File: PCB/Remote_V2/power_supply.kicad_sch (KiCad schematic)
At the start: 69 parts, among them J1 USB_C_Receptacle_USB2.0_16P, J5 USB_C_Receptacle_USB2.0_16P, J6 USB_C_Receptacle_USB2.0_16P, Q1 AO3401A, Q2 AO3401A, Q3 AO3401A, U1 AMS1117-3.3, U3 AMS1117-3.3, U4 AMS1117-3.3, U5 AMS1117-3.3, U7 AMS1117-3.3, U9 AMS1117-3.3

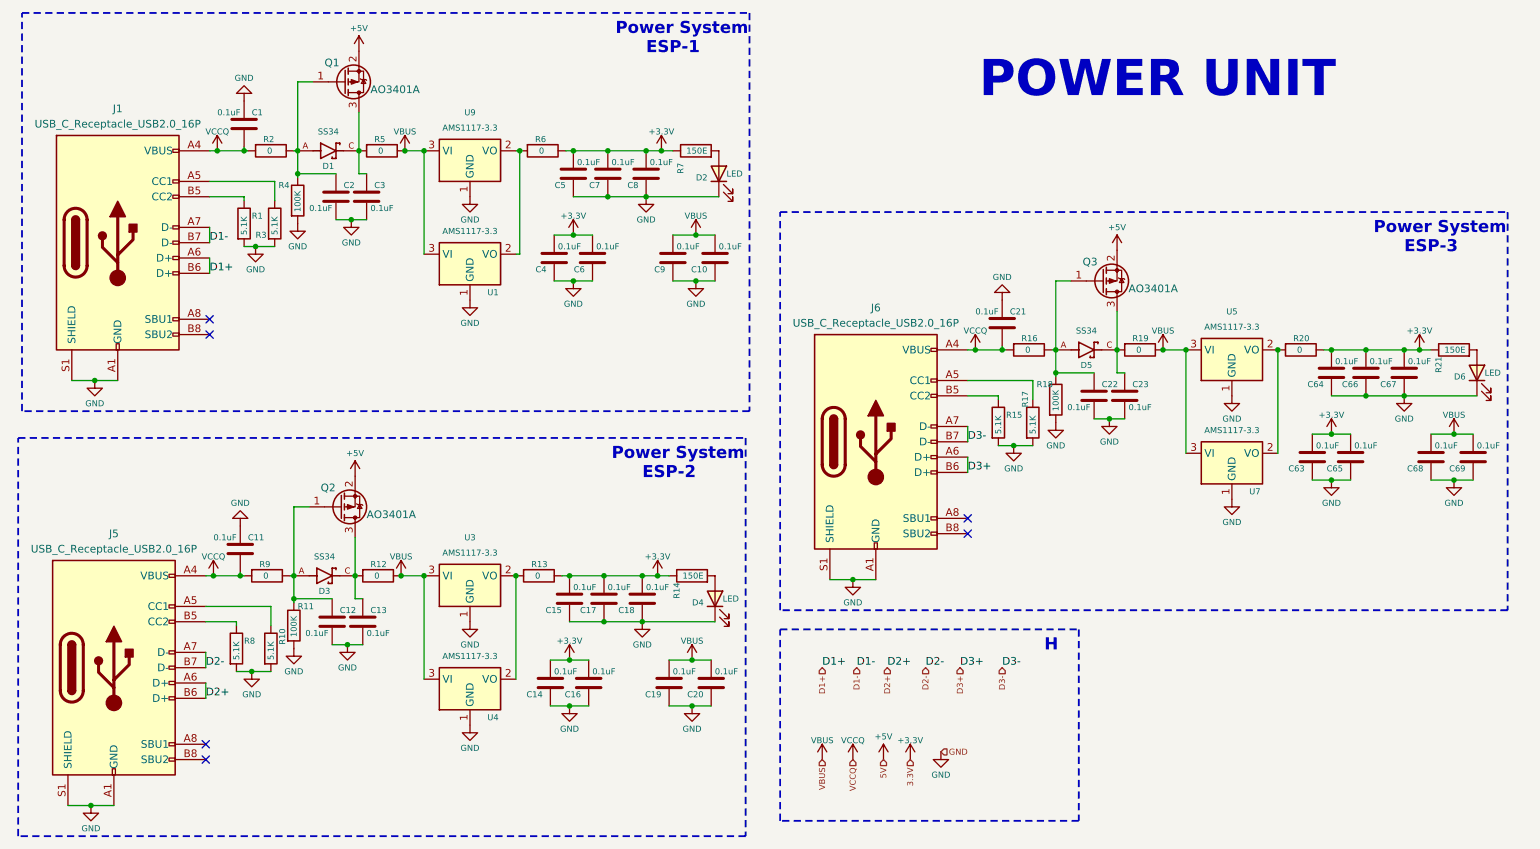
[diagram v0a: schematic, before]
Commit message: update watch_v3
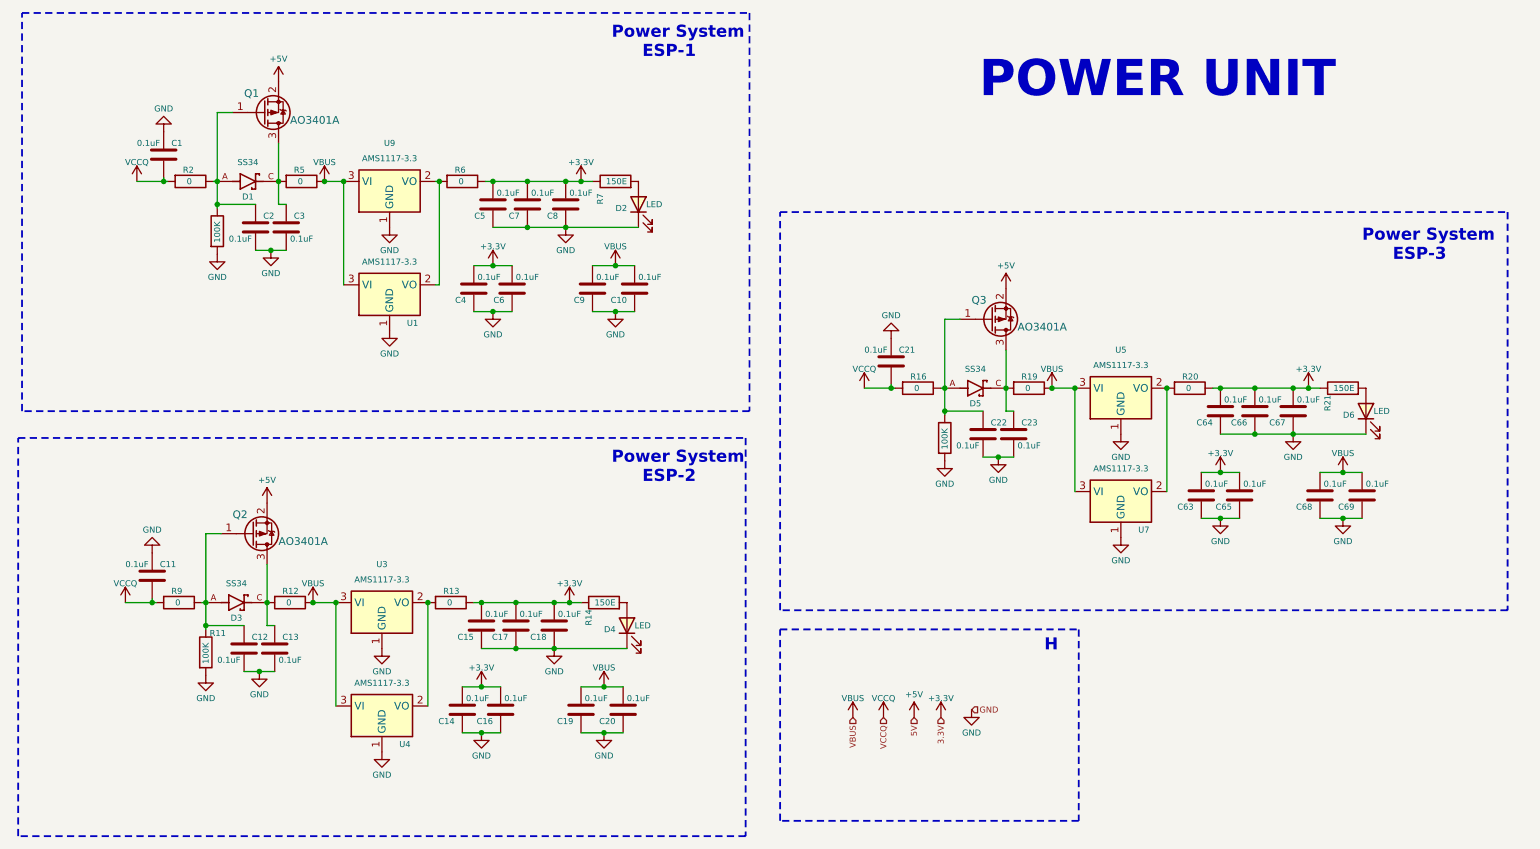
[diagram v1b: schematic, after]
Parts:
- removed J1, J5, J6: USB_C_Receptacle_USB2.0_16P, Connector_USB:USB_C_Receptacle_GCT_USB4105-xx-A_16P_TopMnt_Horizontal, symbol Connector:USB_C_Receptacle_USB2.0_16P
- removed R1, R10, R15, R17, R3, R8: 5.1K, Resistor_SMD:R_0402_1005Metric, symbol Device:R
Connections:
- no-connect marks 6 -> 0
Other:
- moved on the sheet: C1, C10, C11, C12, C13, C14, C15, C16, C17, C18, C19, C2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

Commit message: updating PCBs
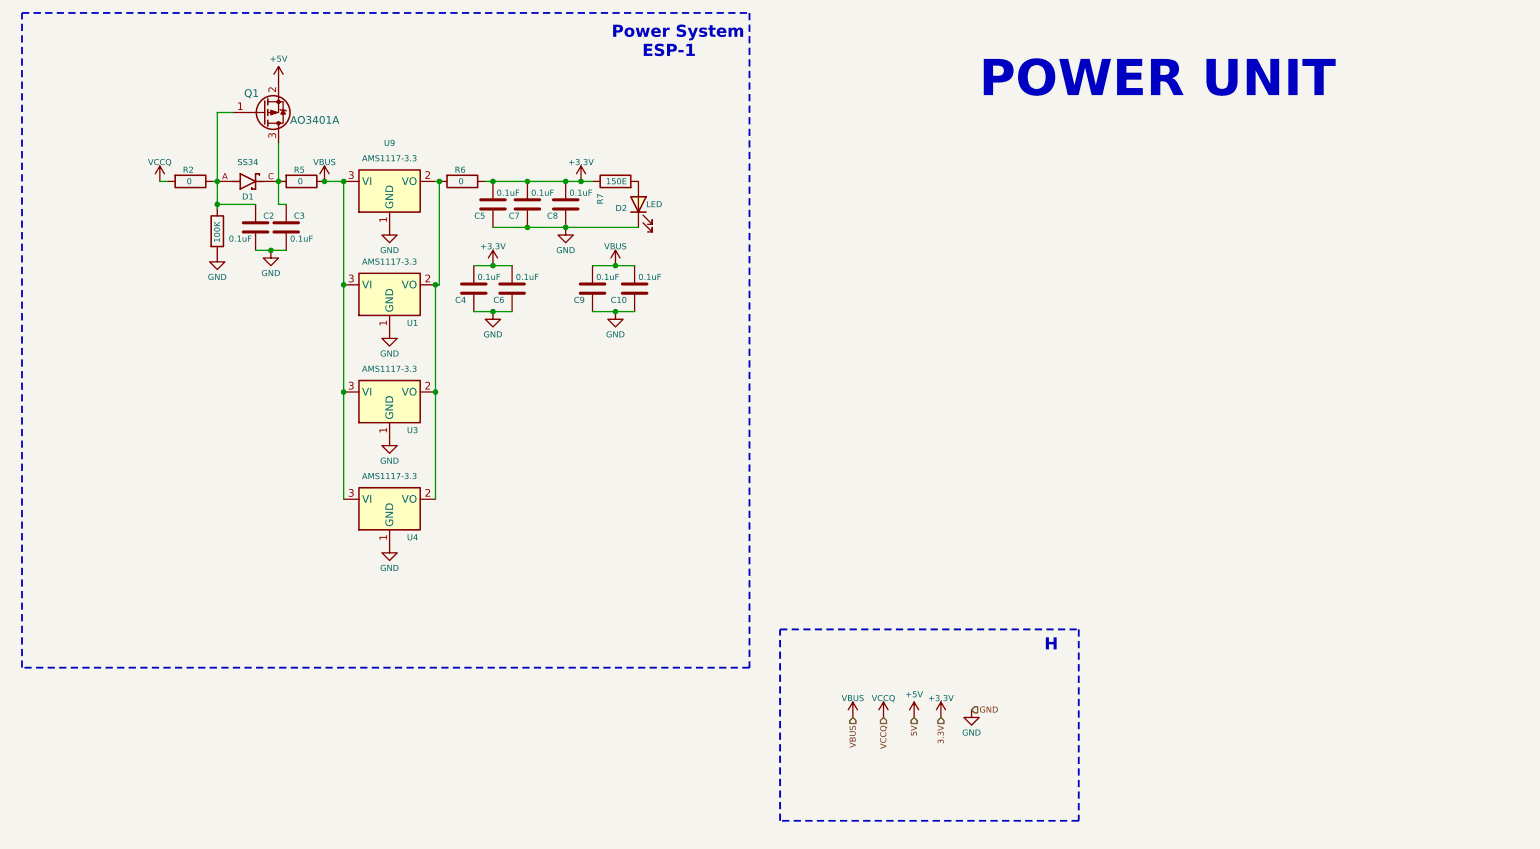
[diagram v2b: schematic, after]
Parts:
- removed C1, C11, C12, C13, C14, C15, C16, C17, C18, C19, C20, C21, C22, C23, C63, C64, C65, C66, C67, C68, C69: 0.1uF, Capacitor_SMD:C_0402_1005Metric, symbol Device:C
- removed D3, D5: SS34, Button_Switch_SMD:P25_DO-214AC_SMA, symbol SS34:SS34
- removed D4, D6: LED, LED_SMD:LED_0402_1005Metric, symbol Device:LED
- removed Q2, Q3: AO3401A, Package_TO_SOT_SMD:SOT-23, symbol Transistor_FET:AO3401A
- removed R11, R18: 100K, Resistor_SMD:R_0402_1005Metric, symbol Device:R
- removed R12, R13, R16, R19, R20, R9: 0, Resistor_SMD:R_0402_1005Metric, symbol Device:R
- removed R14, R21: 150E, Resistor_SMD:R_0402_1005Metric, symbol Device:R
- removed U5, U7: AMS1117-3.3, Package_TO_SOT_SMD:SOT-223-3_TabPin2, symbol Regulator_Linear:AMS1117-3.3
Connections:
- net at U3.2 (VO), U4.2 (VO): now also R6.2, U1.2 (VO), U9.2 (VO)
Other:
- note removed: "ESP-2"
- note removed: "ESP-3"
